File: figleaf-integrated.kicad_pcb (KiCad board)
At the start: 2 copper layers, 145 x 106 mm, 70 parts, among them J1 Conn_01x02_Pin, J2 HRO_TYPE-C-31-M-14, J3 Battery, J9 TC2030_SWD, Q2 2N7002, SW1 PWR, SW2 RST, U1 SRV05-4, U10 MAX17048, U3 BQ24075, U8 nRF52840_moko_mk08

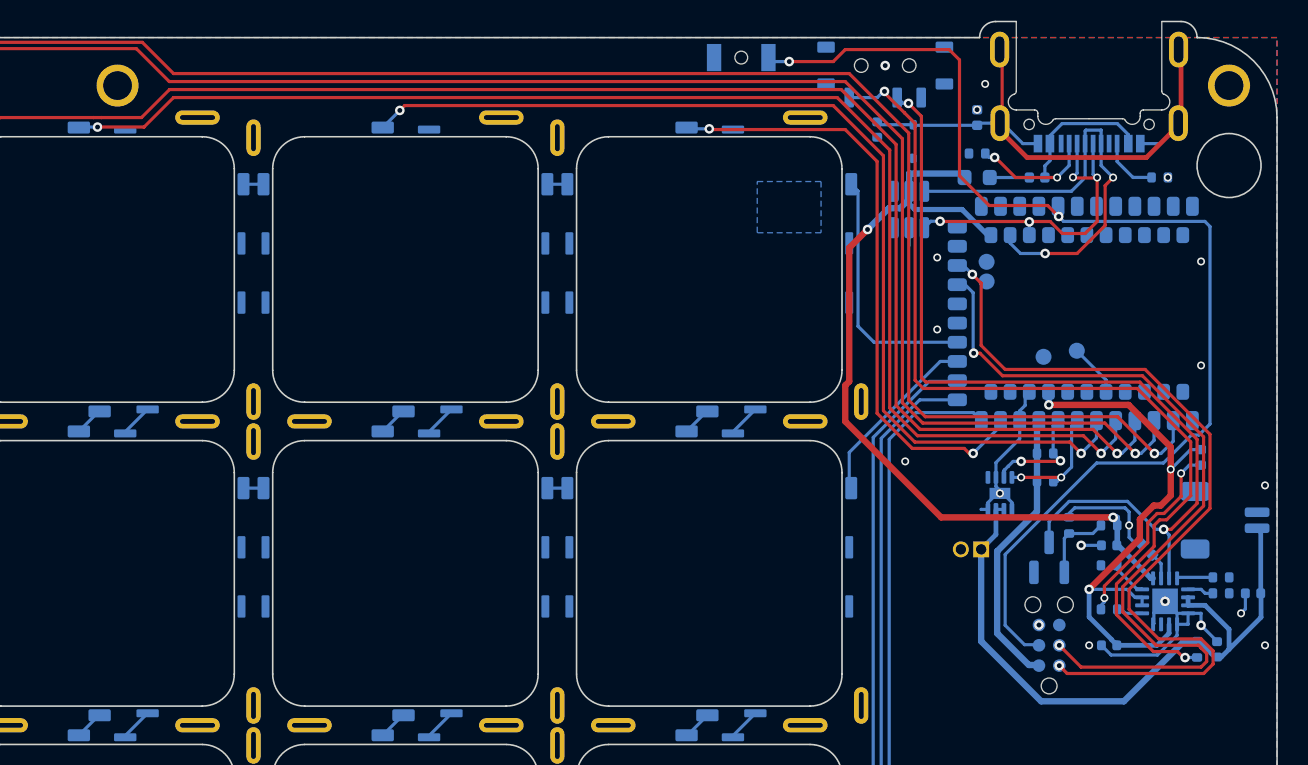
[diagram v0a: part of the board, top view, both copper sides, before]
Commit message: small deets
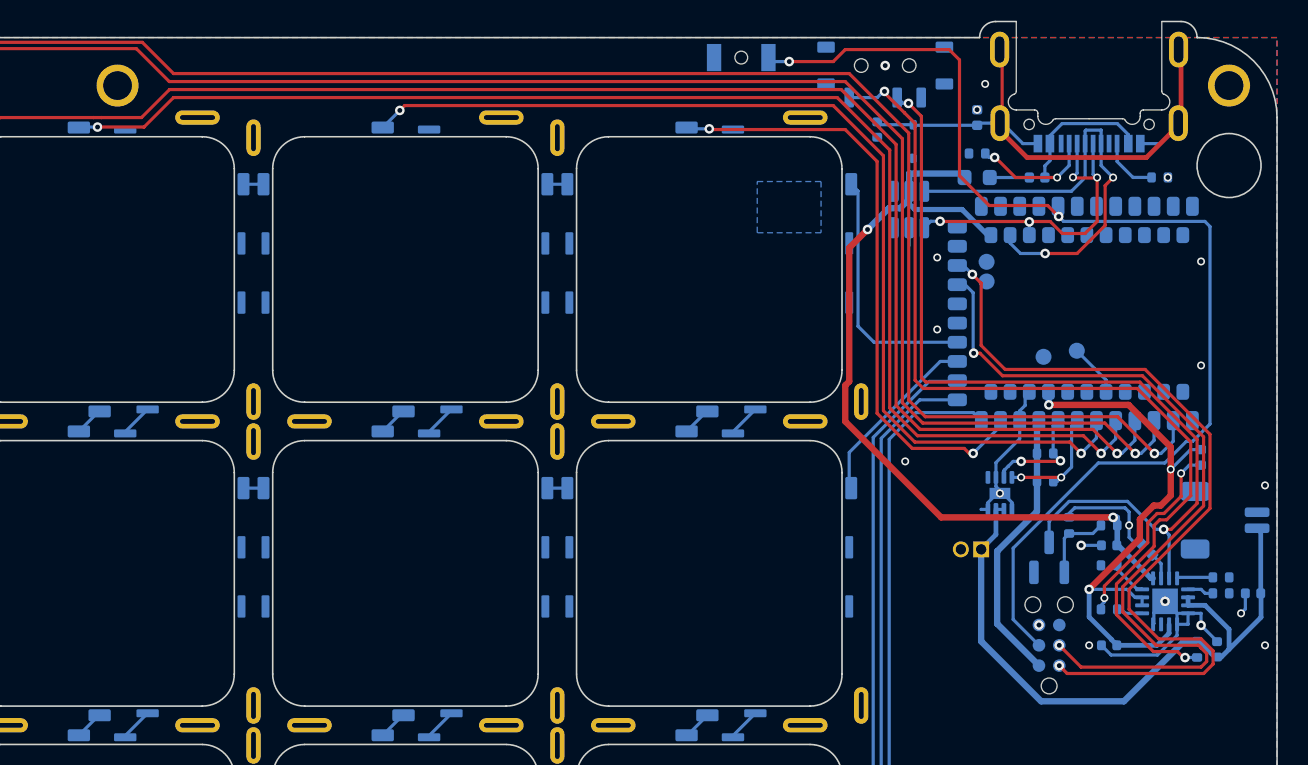
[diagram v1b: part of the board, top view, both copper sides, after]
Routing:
- net RST: track 73.1 -> 72.1 mm
